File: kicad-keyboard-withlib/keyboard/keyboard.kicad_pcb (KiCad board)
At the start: 2 copper layers, 200.5 x 128.5 mm, 47 parts, among them SW1 SW_Push, SW10 SW_Push, SW11 SW_Push, SW12 SW_Push, SW13 SW_Push, SW14 SW_Push, SW15 SW_Push, SW16 SW_Push, SW17 SW_Push, SW18 SW_Push, SW19 SW_Push, SW2 SW_Push, SW20 SW_Push, SW21 SW_Push, SW22 SW_Push, SW23 SW_Push, SW24 SW_Push, SW25 SW_Push, SW26 SW_Push, SW27 SW_Push, SW28 SW_Push, SW29 SW_Push, SW3 SW_Push, SW30 SW_Push, SW31 SW_Push, SW32 SW_Push, SW33 SW_Push, SW34 SW_Push, SW35 SW_Push, SW36 SW_Push, SW37 SW_Push, SW38 SW_Push, SW39 SW_Slide_DPDT, SW4 SW_Push, SW41 RotaryEncoder_Switch, SW5 SW_Push, SW6 SW_Push, SW7 SW_Push, SW8 SW_Push, SW9 SW_Push, U2 MCP23017_SO

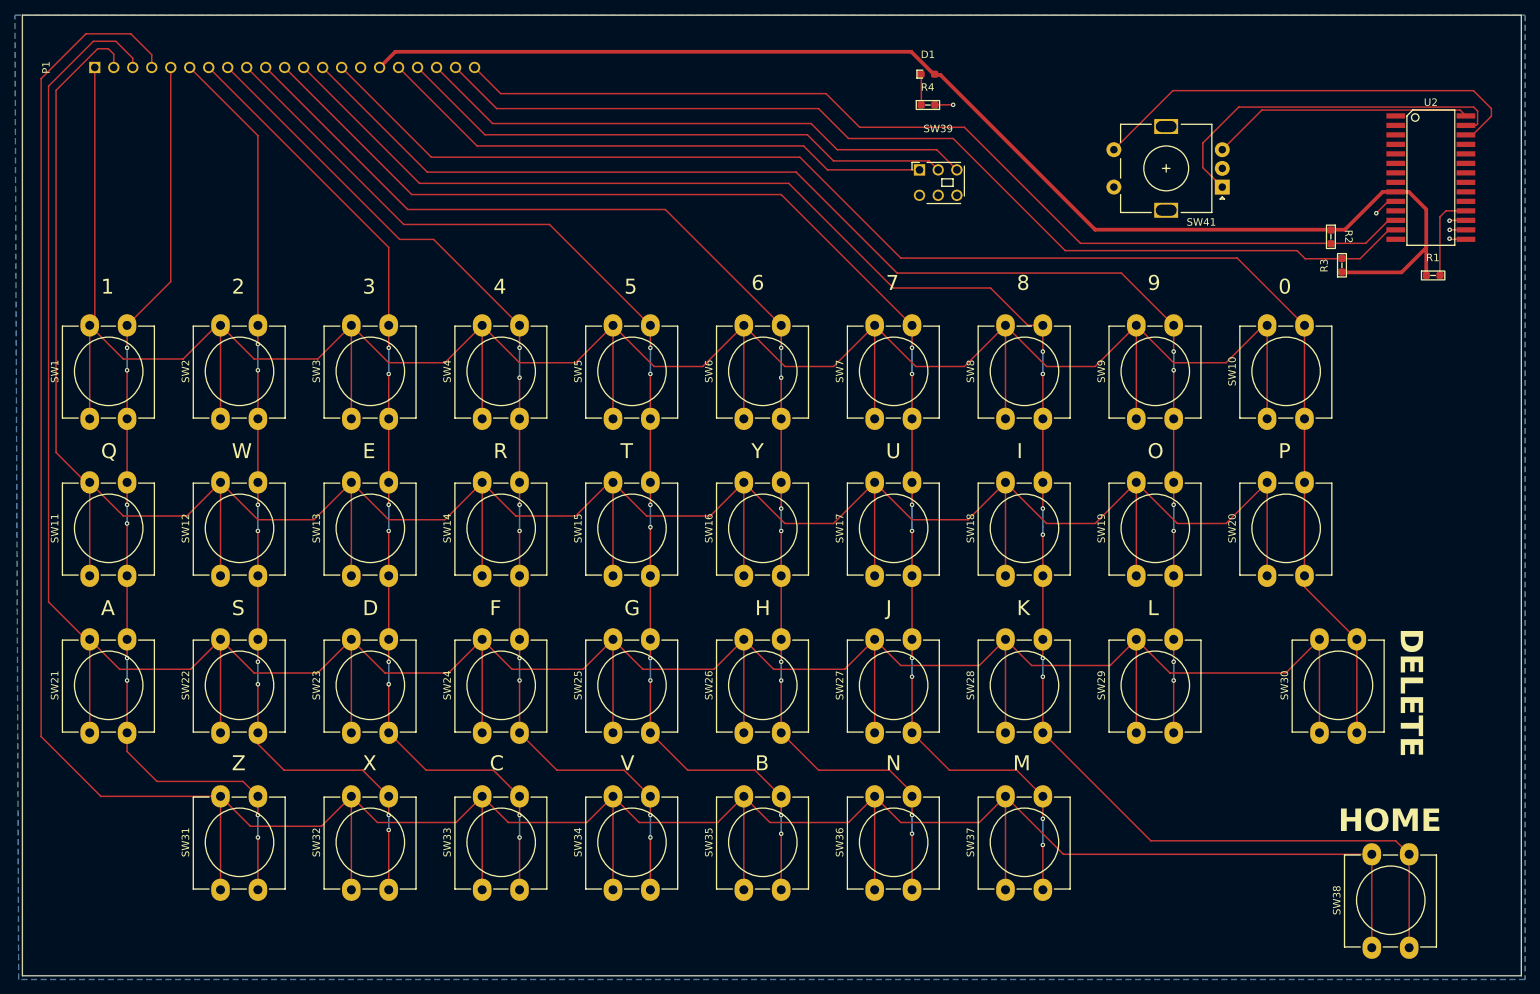
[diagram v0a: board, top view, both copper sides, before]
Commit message: add: all footprint done, pcb with own footprint, to finish
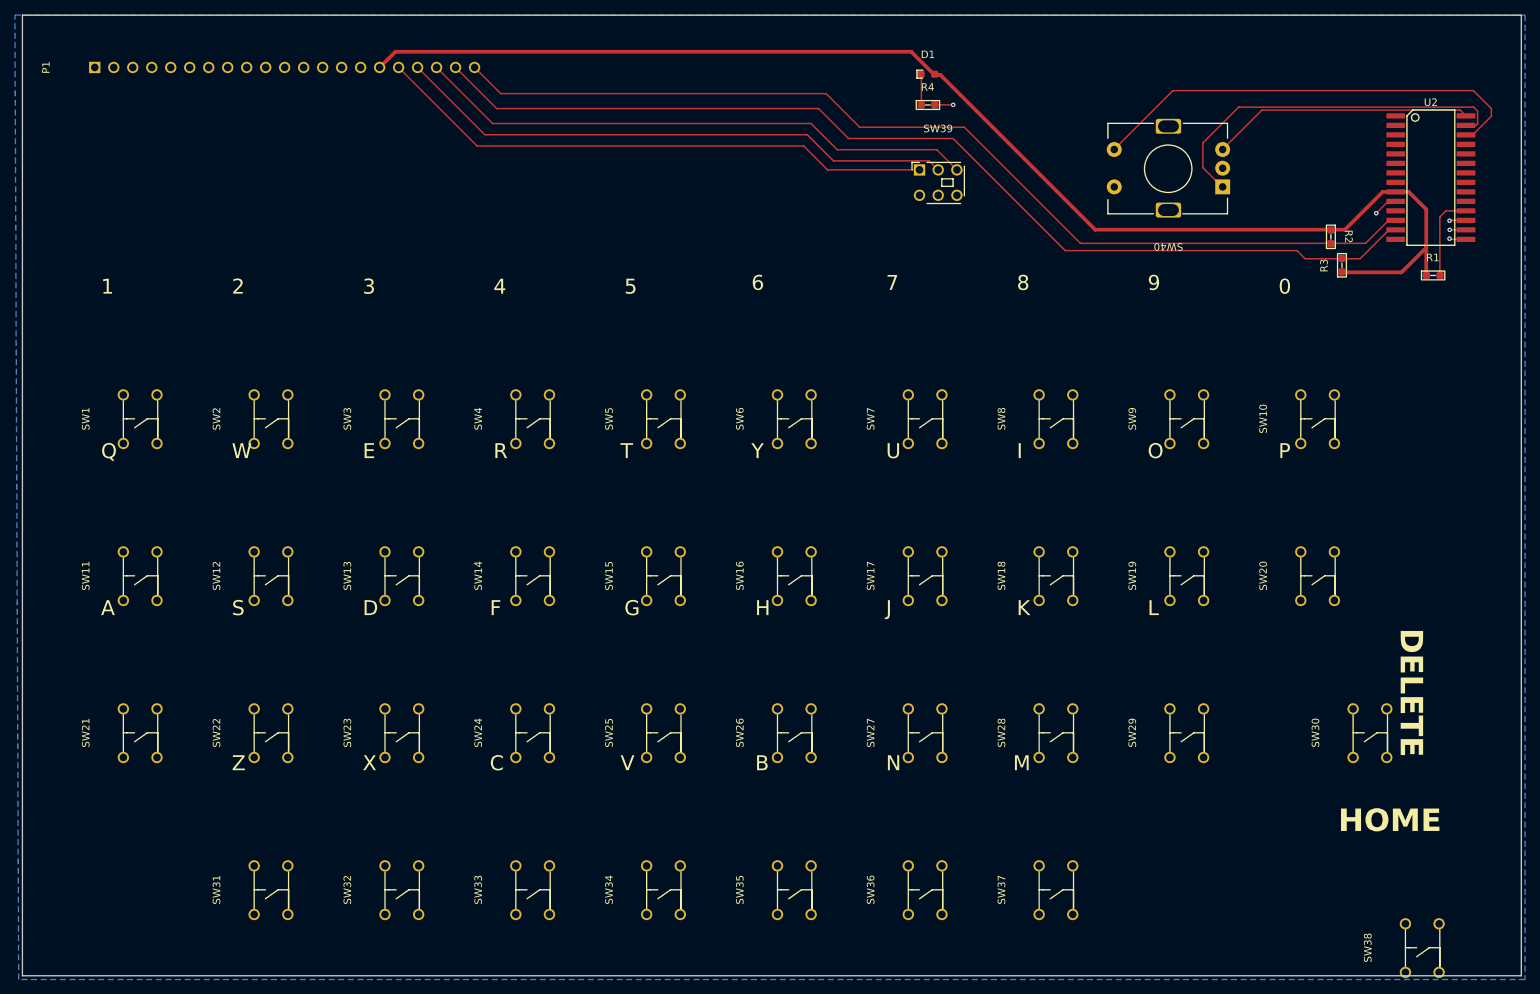
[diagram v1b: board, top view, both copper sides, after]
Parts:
- removed SW41: RotaryEncoder_Switch, Rotary_Encoder:RotaryEncoder_Alps_EC11E-Switch_Vertical_H20mm
- added SW40: ~, Lilyspad:rotary_encoder, F.Cu at (177.8, 66.0)
- SW1, SW10, SW11, SW12, SW13, SW14, SW15, SW16, SW17, SW18, SW19, SW2, SW20, SW21, SW22, SW23, SW24, SW25, SW26, SW27, SW28, SW29, SW3, SW30, SW31, SW32, SW33, SW34, SW35, SW36, SW37, SW38, SW4, SW5, SW6, SW7, SW8, SW9: footprint Button_Switch_THT:SW_PUSH-12mm_Wuerth-430476085716 -> Lilyspad:push_switch
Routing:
- net Net-(P1-R3): track 412.2 -> 0.00 mm
- net Net-(P1-R4): track 410.5 -> 0.00 mm
- net Net-(P1-R2): track 386.5 -> 0.00 mm
- net Net-(P1-R1): track 355.4 -> 0.00 mm
- net Net-(P1-C8): track 235.9 -> 0.00 mm, vias 6 -> 0
- net Net-(P1-C10): track 200.5 -> 0.00 mm
- net Net-(P1-C7): track 186.2 -> 0.00 mm, vias 8 -> 0
- net Net-(P1-C9): track 182.6 -> 0.00 mm, vias 6 -> 0
- net Net-(P1-C6): track 171.6 -> 0.00 mm, vias 8 -> 0
- net Net-(P1-C5): track 156.3 -> 0.00 mm, vias 8 -> 0
- net Net-(P1-C4): track 141.4 -> 0.00 mm, vias 8 -> 0
- net Net-(P1-C3): track 132.5 -> 0.00 mm, vias 8 -> 0
- net Net-(P1-C2): track 127.2 -> 0.00 mm, vias 8 -> 0
- net Net-(P1-C1): track 126.4 -> 0.00 mm, vias 8 -> 0
